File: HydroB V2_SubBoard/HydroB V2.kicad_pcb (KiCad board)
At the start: 4 copper layers, 106.8 x 81.2 mm, 122 parts, among them J10 Screw_Terminal_01x02, J16 Screw_Terminal_01x02, J3 Screw_Terminal_01x02, J4 Conn_01x04_Pin, J5 PH SENSOR, J6 EC SENSOR, J7 Conn_01x02_Pin, J8 Screw_Terminal_01x02, J9 Screw_Terminal_01x02, Q1 S8050, Q2 S8050, Q3 S8050, Q4 S8050, Q5 S8050, SW1 SW_Push, U1 STM32F103C8Tx, U3 SN65HVD72DR, U4 LMR33620ADDA, Y1 8Mhz

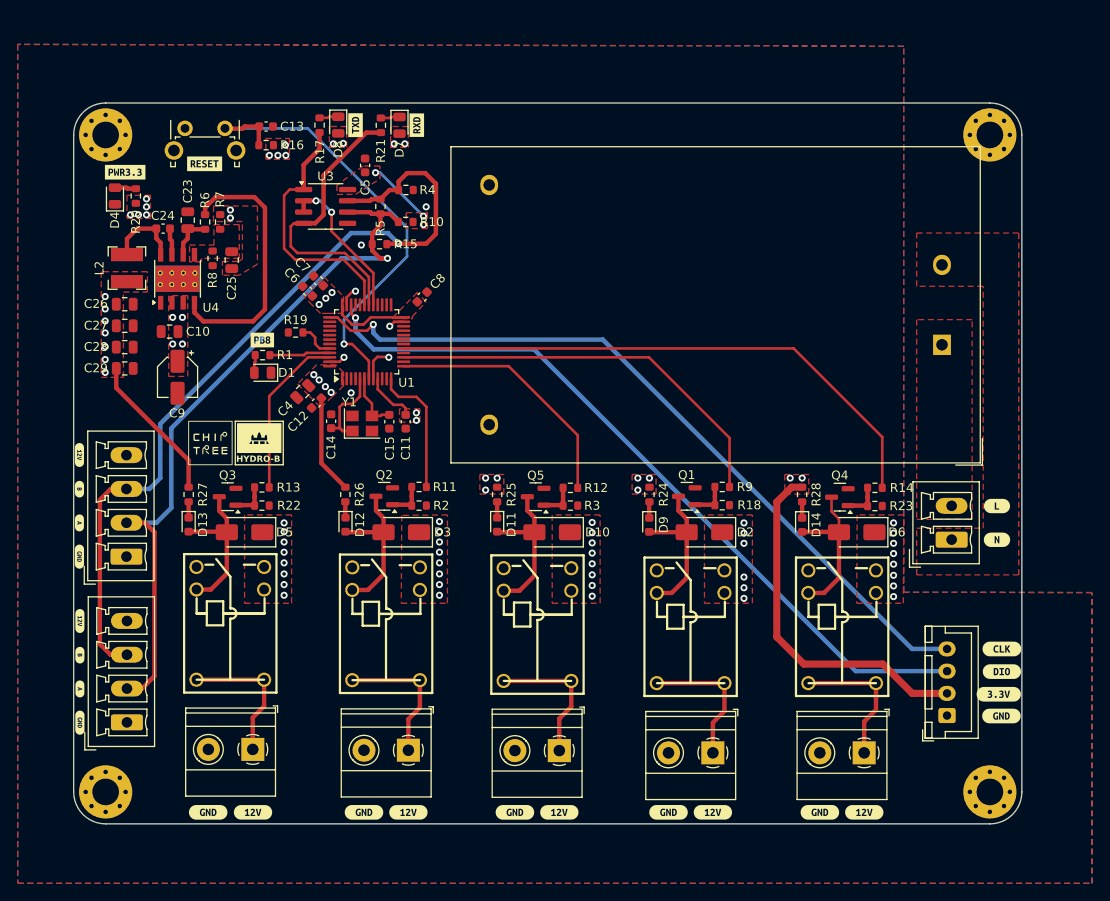
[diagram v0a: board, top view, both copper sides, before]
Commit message: PCB update
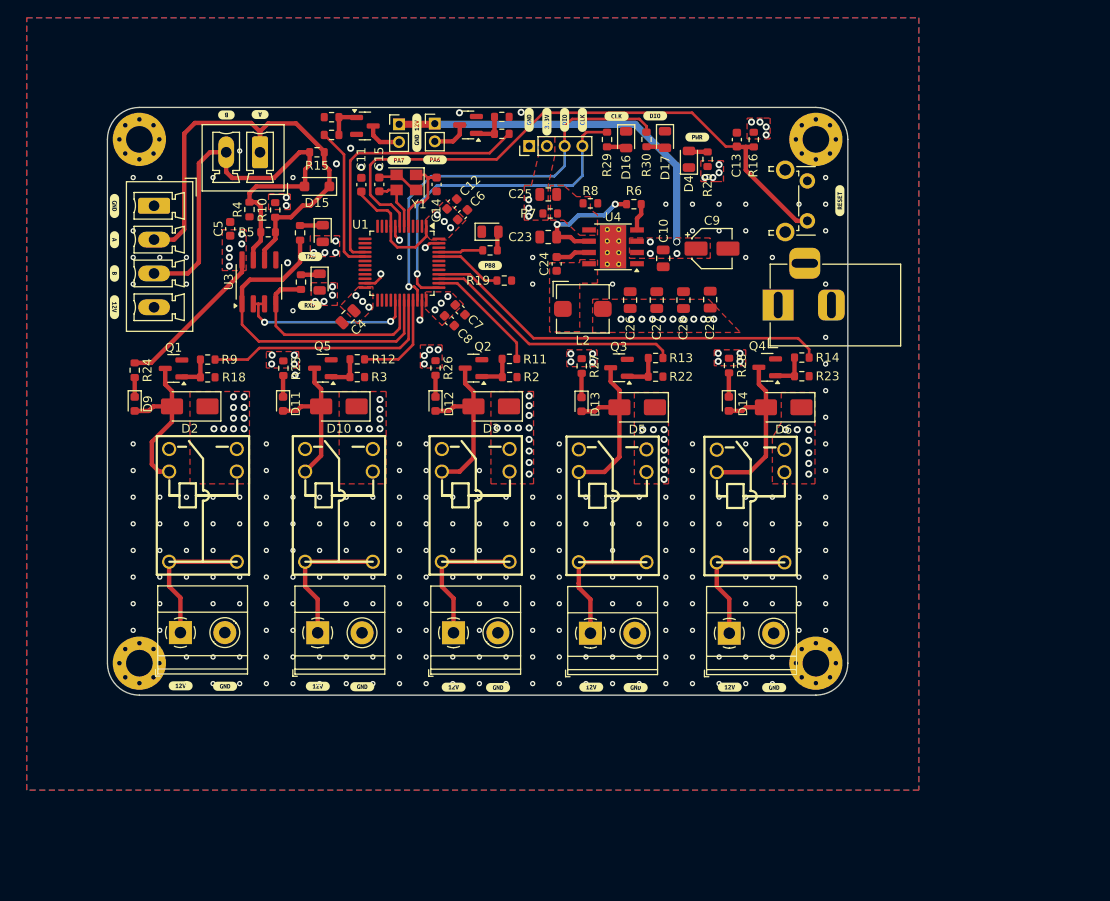
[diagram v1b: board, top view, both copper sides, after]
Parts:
- removed G***: LOGO, CHIPTREE_LOGO:cam5x5
- removed G***: LOGO, CHIPTREE_LOGO:CHPTREE-5x5mm
- removed PS2: HLK-20M12, Converter_ACDC:Converter_ACDC_Hi-Link_HLK-20Mxx
- removed kibuzzard-668BA666: G***, kibuzzard-668BA666
- removed kibuzzard-668BA6B4: G***, kibuzzard-668BA6B4
- removed kibuzzard-668BA6C7: G***, kibuzzard-668BA6C7
- removed kibuzzard-668BA6F1: G***, kibuzzard-668BA6F1
- removed kibuzzard-668BA7A5: G***, kibuzzard-668BA7A5
- removed kibuzzard-668BA7C8: G***, kibuzzard-668BA7C8
- removed kibuzzard-668BA7EF: G***, kibuzzard-668BA7EF
- removed kibuzzard-668BA811: G***, kibuzzard-668BA811
- removed kibuzzard-668BA833: G***, kibuzzard-668BA833
- removed kibuzzard-668BA852: G***, kibuzzard-668BA852
- removed kibuzzard-668BA86D: G***, kibuzzard-668BA86D
- removed kibuzzard-668BA998 (x2): G***, kibuzzard-668BA998
- removed kibuzzard-668BA9FB (x2): G***, kibuzzard-668BA9FB
- removed kibuzzard-668BAA24 (x2): G***, kibuzzard-668BAA24
- removed kibuzzard-668BAA39 (x2): G***, kibuzzard-668BAA39
- removed kibuzzard-668BAA96 (x5): G***, kibuzzard-668BAA96
- removed kibuzzard-668BAD03 (x5): G***, kibuzzard-668BAD03
- added D15: D_TVS, Diode_SMD:D_SOD-123F, F.Cu at (124.2, 65.0)
- added D16: LED_Small, LED_SMD:LED_0805_2012Metric, F.Cu at (159.0, 59.7)
- added D17: LED_Small, LED_SMD:LED_0805_2012Metric, F.Cu at (163.4, 59.7)
- added J1: Conn_01x02_Pin, Connector_Phoenix_MC:PhoenixContact_MCV_1,5_2-G-3.81_1x02_P3.81mm_Vertical, F.Cu at (117.8, 61.1)
- added J2: 12V, Connector_BarrelJack:BarrelJack_Horizontal, F.Cu at (176.2, 78.4)
- added Q6: S8050, Package_TO_SOT_SMD:SOT-23, F.Cu at (129.6, 58.2)
- added Q7: S8050, Package_TO_SOT_SMD:SOT-23, F.Cu at (141.2, 58.1)
- added R29: 1k, Resistor_SMD:R_0603_1608Metric, F.Cu at (156.9, 59.7)
- added R30: 1k, Resistor_SMD:R_0603_1608Metric, F.Cu at (161.3, 59.7)
- added R31: 1K, Resistor_SMD:R_0603_1608Metric, F.Cu at (125.8, 59.2)
- added R32: 10K, Resistor_SMD:R_0603_1608Metric, F.Cu at (125.8, 57.2)
- added R33: 1K, Resistor_SMD:R_0603_1608Metric, F.Cu at (145.0, 59.1)
- added R34: 10K, Resistor_SMD:R_0603_1608Metric, F.Cu at (145.0, 57.2)
- added kibuzzard-669F2037: G***, kibuzzard-669F2037, F.Cu at (135.4, 59.0)
- added kibuzzard-669F208D: G***, kibuzzard-669F208D, F.Cu at (137.5, 62.0)
- added kibuzzard-669F20C5: G***, kibuzzard-669F20C5, F.Cu at (133.4, 62.0)
- added kibuzzard-669F20DD: G***, kibuzzard-669F20DD, F.Cu at (148.1, 57.5)
- added kibuzzard-669F20FF: G***, kibuzzard-669F20FF, F.Cu at (150.1, 57.7)
- added kibuzzard-669F211D: G***, kibuzzard-669F211D, F.Cu at (152.1, 57.5)
- added kibuzzard-669F2125: G***, kibuzzard-669F2125, F.Cu at (154.1, 57.5)
- added kibuzzard-669F24DA: G***, kibuzzard-669F24DA, F.Cu at (157.9, 57.1)
- added kibuzzard-669F24EA: G***, kibuzzard-669F24EA, F.Cu at (162.3, 57.0)
- added kibuzzard-669F2500: G***, kibuzzard-669F2500, F.Cu at (167.0, 59.5)
- added kibuzzard-669F250D: G***, kibuzzard-669F250D, F.Cu at (183.1, 66.6)
- added kibuzzard-669F251A: G***, kibuzzard-669F251A, F.Cu at (143.7, 73.9)
- added kibuzzard-669F255D: G***, kibuzzard-669F255D, F.Cu at (123.5, 72.9)
- added kibuzzard-669F2571: G***, kibuzzard-669F2571, F.Cu at (123.4, 78.4)
- added kibuzzard-669F2588: G***, kibuzzard-669F2588, F.Cu at (117.8, 56.9)
- added kibuzzard-669F2592: G***, kibuzzard-669F2592, F.Cu at (114.0, 57.0)
- added kibuzzard-669F259B: G***, kibuzzard-669F259B, F.Cu at (101.4, 67.2)
- added kibuzzard-669F25AE: G***, kibuzzard-669F25AE, F.Cu at (101.4, 71.0)
- added kibuzzard-669F25B6: G***, kibuzzard-669F25B6, F.Cu at (101.4, 74.8)
- added kibuzzard-669F25BD: G***, kibuzzard-669F25BD, F.Cu at (101.4, 78.6)
- added kibuzzard-669F25C8: G***, kibuzzard-669F25C8, F.Cu at (108.8, 121.2)
- added kibuzzard-669F25D3: G***, kibuzzard-669F25D3, F.Cu at (113.8, 121.3)
- added kibuzzard-669F25DA: G***, kibuzzard-669F25DA, F.Cu at (124.3, 121.3)
- added kibuzzard-669F25E1: G***, kibuzzard-669F25E1, F.Cu at (129.3, 121.3)
- added kibuzzard-669F25EE: G***, kibuzzard-669F25EE, F.Cu at (139.6, 121.4)
- added kibuzzard-669F25F4: G***, kibuzzard-669F25F4, F.Cu at (144.6, 121.5)
- added kibuzzard-669F25FE: G***, kibuzzard-669F25FE, F.Cu at (155.1, 121.4)
- added kibuzzard-669F2610: G***, kibuzzard-669F2610, F.Cu at (160.1, 121.5)
- added kibuzzard-669F261C: G***, kibuzzard-669F261C, F.Cu at (170.7, 121.4)
- added kibuzzard-669F2622: G***, kibuzzard-669F2622, F.Cu at (175.7, 121.5)
- J4: footprint Connector_JST:JST_XH_B4B-XH-A_1x04_P2.50mm_Vertical -> Connector_PinHeader_2.00mm:PinHeader_1x04_P2.00mm_Vertical
- J5: value PH SENSOR -> Conn_01x02_Pin; footprint Connector_Phoenix_MC:PhoenixContact_MCV_1,5_4-G-3.81_1x04_P3.81mm_Vertical -> Connector_PinHeader_2.00mm:PinHeader_1x02_P2.00mm_Vertical
- J6: value EC SENSOR -> SENSOR
- J7: footprint Connector_Phoenix_MC:PhoenixContact_MCV_1,5_2-G-3.81_1x02_P3.81mm_Vertical -> Connector_PinHeader_2.00mm:PinHeader_1x02_P2.00mm_Vertical
- L2: footprint Inductor_SMD:L_Bourns-SRN4018 -> Inductor_SMD:L_Bourns_SRP5030T
- moved H6 120.7 mm to (104.2, 59.7)
- moved H8 99.7 mm to (180.4, 118.7)
- moved J4 79.6 mm to (148.1, 60.5)
- moved J7 74.7 mm to (137.5, 57.9), turned to 0 degrees
- moved SW1 70.3 mm to (179.4, 64.4), turned to -90 degrees
- moved C29 66.4 mm to (168.5, 77.8), turned to 90 degrees
- moved D4 64.8 mm to (166.1, 61.9)
- moved R20 64.5 mm to (168.2, 61.9)
- moved C28 63.2 mm to (165.5, 77.8), turned to 90 degrees
- moved C9 61.9 mm to (168.7, 72.0), turned to 0 degrees
- moved J3 61.5 mm to (108.8, 115.3), turned to 0 degrees
- moved C27 60.0 mm to (162.5, 77.8), turned to 90 degrees
- moved R18 59.7 mm to (111.9, 86.5)
- moved R9 59.7 mm to (111.9, 84.5)
- moved D2 59.7 mm to (109.9, 89.8)
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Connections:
- J5 pad 1: GND -> +12V
- J6 pad 2: Net-(J5-Pin_2) -> Net-(D15-A1)
- J6 pad 3: Net-(J5-Pin_3) -> Net-(D15-A2)
- J7 pad 1: N -> +12V
- J7 pad 2: L -> Net-(J7-Pin_2)
- R10 pad 2: Net-(J5-Pin_2) -> Net-(D15-A1)
- R15 pad 1: Net-(J5-Pin_2) -> Net-(D15-A1)
- R15 pad 2: Net-(J5-Pin_3) -> Net-(D15-A2)
- R4 pad 1: Net-(J5-Pin_3) -> Net-(D15-A2)
- R5 pad 1: Net-(J5-Pin_2) -> Net-(D15-A1)
- R5 pad 2: Net-(J5-Pin_3) -> Net-(D15-A2)
- U1 pad 12: /HydroB/Block Relay1/RELAY_3 -> unconnected-(U1-PA2-Pad12)
- U1 pad 13: /HydroB/Block Relay1/RELAY_2 -> unconnected-(U1-PA3-Pad13)
- U1 pad 15: /HydroB/Block Relay1/RELAY_1 -> unconnected-(U1-PA5-Pad15)
- U1 pad 16: unconnected-(U1-PA6-Pad16) -> LED2
- U1 pad 17: /HydroB/Block Relay1/RELAY_5 -> LED1
- U1 pad 32: unconnected-(U1-PA11-Pad32) -> /HydroB/Block Relay1/RELAY_1
- U1 pad 33: unconnected-(U1-PA12-Pad33) -> /HydroB/Block Relay1/RELAY_2
- U1 pad 38: unconnected-(U1-PA15-Pad38) -> /HydroB/Block Relay1/RELAY_3
- U1 pad 39: unconnected-(U1-PB3-Pad39) -> /HydroB/Block Relay1/RELAY_4
- U1 pad 40: unconnected-(U1-PB4-Pad40) -> /HydroB/Block Relay1/RELAY_5
- U1 pad 46: /HydroB/Block Relay1/RELAY_4 -> unconnected-(U1-PB9-Pad46)
- U3 pad 6: Net-(J5-Pin_2) -> Net-(D15-A1)
- U3 pad 7: Net-(J5-Pin_3) -> Net-(D15-A2)
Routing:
- net Net-(J5-Pin_3): track 93.9 -> 0.00 mm, vias 1 -> 0
- net Net-(J5-Pin_2): track 83.3 -> 4.28 mm, vias 1 -> 0
- net +3.3V: track 90.6 -> 31.3 mm, vias 42 -> 61
- net Net-(D15-A1): track 0.00 -> 54.8 mm
- net Net-(D15-A2): track 0.00 -> 52.8 mm
- net SWCLK: track 86.1 -> 38.9 mm
- net +12V: track 0.00 -> 41.1 mm, vias 42 -> 46
- net SWDIO: track 85.7 -> 46.3 mm
- net LED2: track 0.00 -> 30.9 mm
- net PG: track 30.0 -> 3.10 mm
- net /HydroB/Block Relay1/RELAY_1: track 46.0 -> 27.2 mm
- net /HydroB/Block Relay1/RELAY_5: track 63.8 -> 46.1 mm
- net /HydroB/Block Relay1/RELAY_2: track 28.8 -> 11.2 mm
- net LED1: track 0.00 -> 16.7 mm
- net NRST: track 52.9 -> 68.2 mm, vias 1 -> 0
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- added copper zone on F.Cu, net A
- removed copper zone on F.Cu, net L
- removed copper zone on F.Cu, net N
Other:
- board size 106.8 x 81.2 mm -> 83.4 x 66.2 mm
- board text removed: "HYDRO-B"
